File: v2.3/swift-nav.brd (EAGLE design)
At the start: 53 x 53 mm, 151 parts, among them J1 SMA_EDGE, J6 ZX62-B-5PA, Q1 IRLML6401, U1 6SLX9FTG256, U10 MAX2769, U12 PT7M8206B33TA5EX, U13 M25PX80, U2 LTC3407A_DFN, U3 STM32-M-64-LQFP, U4 7Q-16.368MBG-T, U5 SMA_PATCH_SMDGND, U6 93LC56BT-I/OT, U7 FT232HQ, U8 B4050, U9 XC2401, X3 FPGA DEBUG, X4 NX5032GA-12M, X5 CONN_5-2

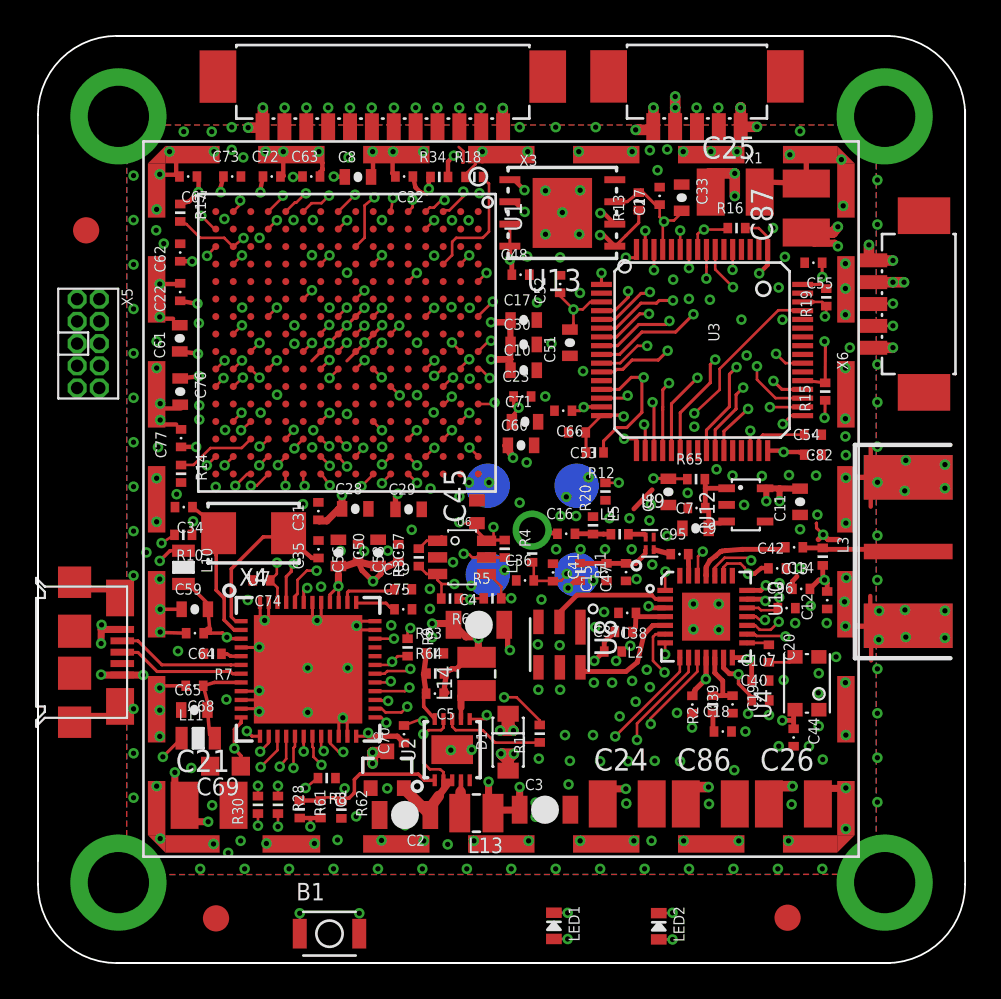
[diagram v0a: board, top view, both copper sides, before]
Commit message: Finished moving stuff around, routing, and DRC. Need to look at soldermask.
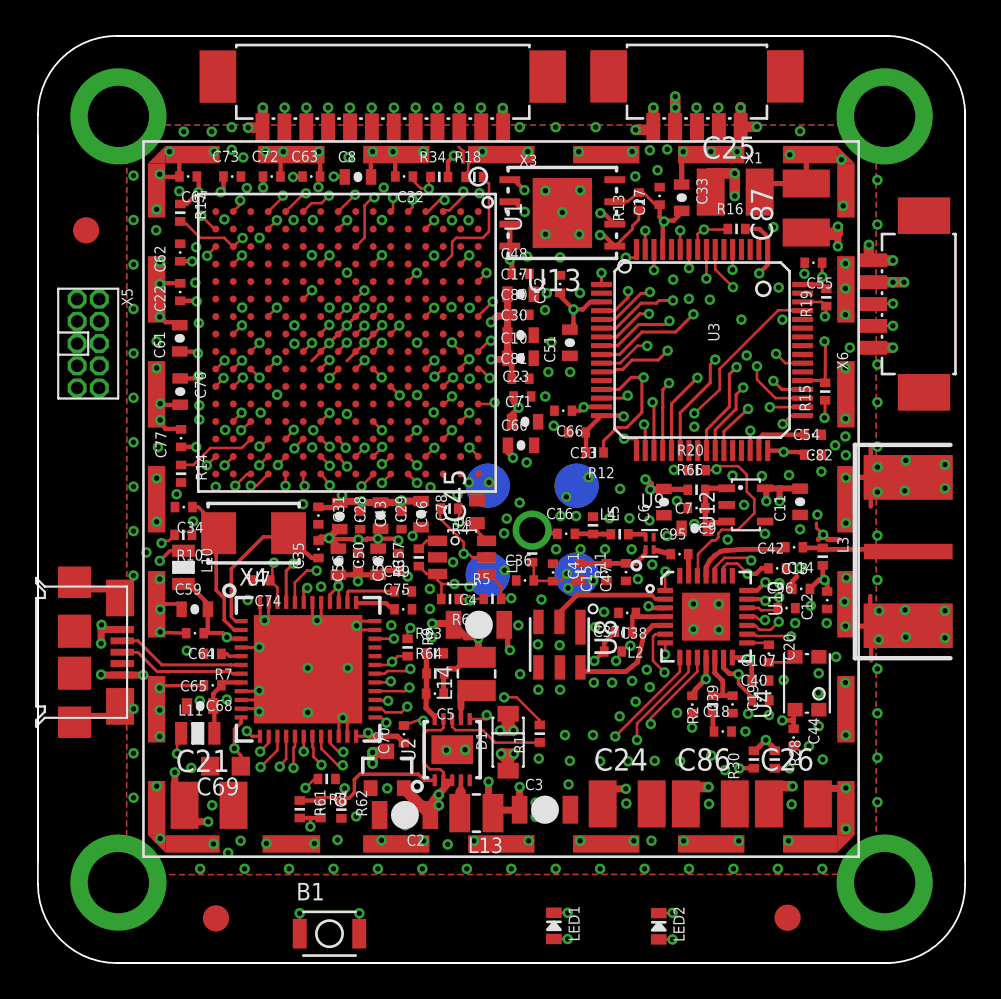
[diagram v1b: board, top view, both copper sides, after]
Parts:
- added C43, C46, C80, C81: 0.47uF, pel_dipol_comp:0402-CAP
- added C78: 4.7uF, pel_dipol_comp:0603-CAP
- moved R28 28.5 mm to (45.5, 15.0)
- moved R30 28.5 mm to (44.3, 15.0)
- moved R20 5.37 mm to (41.1, 31.6), turned to 0 degrees
- moved R4 3.90 mm to (26.9, 29.4), turned to 180 degrees
- moved C29 1.64 mm to (23.0, 29.0), turned to 270 degrees
- moved C17 1.48 mm to (31.0, 41.6)
- moved C68 1.04 mm to (13.4, 19.3)
- moved C28 0.98 mm to (20.7, 29.0), turned to 270 degrees
- moved C10 0.71 mm to (31.0, 38.0)
- moved C6 0.64 mm to (39.2, 29.8)
- moved R65 0.61 mm to (41.0, 30.5)
- moved C30 0.56 mm to (31.0, 39.3)
- moved C56 0.51 mm to (21.7, 26.3)
- moved C57 0.51 mm to (22.8, 26.3)
- moved C58 0.51 mm to (24.0, 26.3)
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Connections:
- net GND: now also C43.P$2, C46.P$2, C78.P$2, C80.P$2, C81.P$2
- net VCCINT: now also C43.P$1, C46.P$1, C78.P$1, C80.P$1, C81.P$1
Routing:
- net VCCINT: track 74.9 -> 49.5 mm, vias 15 -> 16
- net N$55: track 31.2 -> 16.3 mm
- net GND: track 108.3 -> 121.9 mm, vias 315 -> 337
- net JTAG_RST: track 117.2 -> 107.7 mm
- net VDD: track 44.9 -> 54.0 mm, vias 4 -> 6
- net MAX_PGM: track 31.3 -> 23.9 mm, vias 4 -> 2
- net VCCIO: track 166.7 -> 173.8 mm, vias 80 -> 79
- net N$24: track 24.9 -> 18.4 mm
- net FTDI_NRST: track 104.9 -> 100.9 mm
- net FPGA_DONE: track 51.6 -> 49.5 mm
- net N$23: track 15.0 -> 17.1 mm
- net N$18: track 68.5 -> 66.6 mm
- net FTDI_NOE: track 21.2 -> 19.8 mm
- net N$21: track 5.58 -> 4.15 mm
- net N$39: track 87.7 -> 86.5 mm
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- added copper zone on layer 15, net VCCINT
